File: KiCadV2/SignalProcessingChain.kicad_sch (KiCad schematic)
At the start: 29 parts, among them U10 NC7SZ157P6X, U11 NC7SZ157P6X, U12 NC7SZ157P6X, U13 NC7SZ157P6X, U14 74LV08AT14-13, U15 HIP4080A, U17 MX3502S, U8 NC7SZ157P6X, U9 NC7SZ157P6X

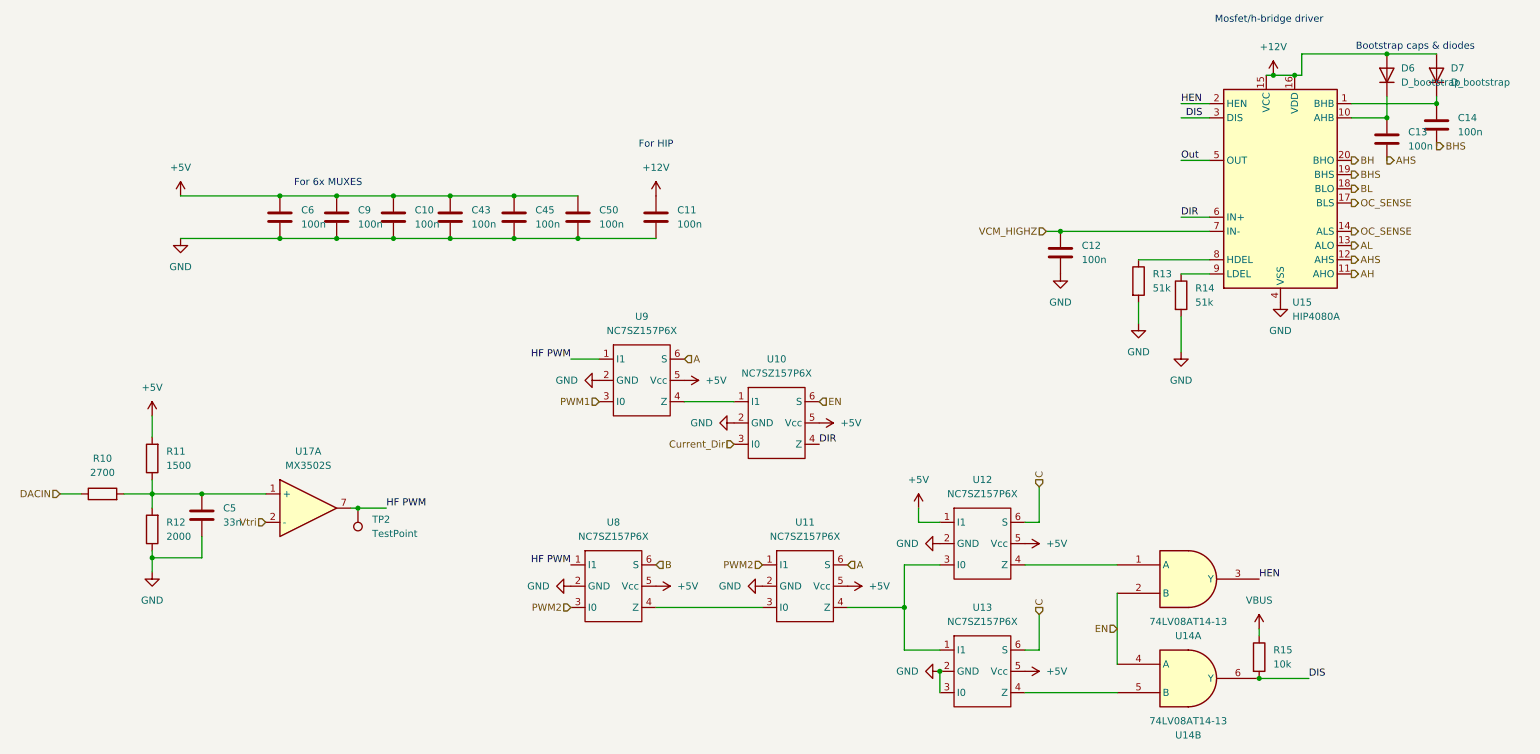
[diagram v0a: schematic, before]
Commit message: saving here before i try making PerCoilFlipped on schematic
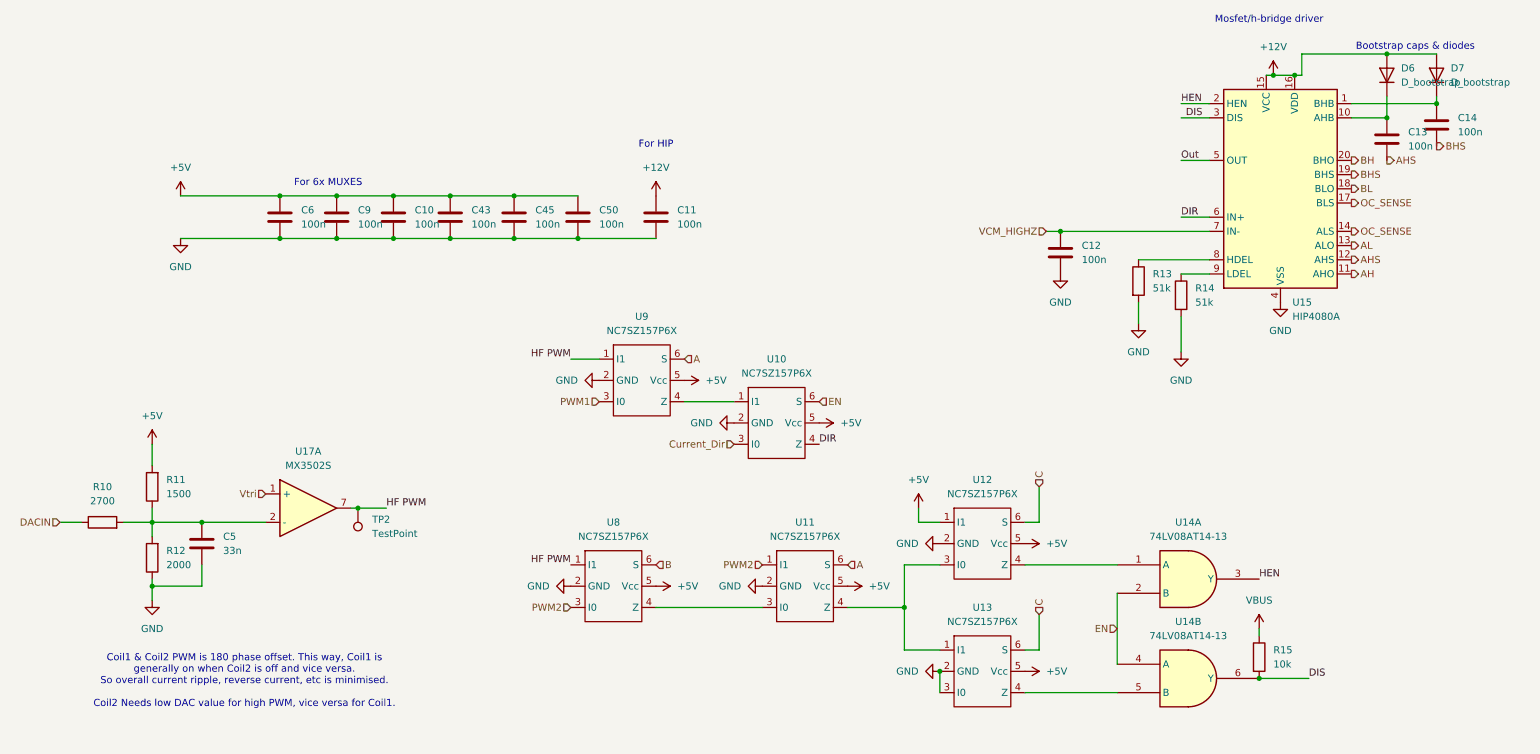
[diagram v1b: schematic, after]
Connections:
- net Vtri: now also U17.1 (+); no longer U17.2 (-)
- net at C5.1, R10.2, R11.1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: now also U17.2 (-); no longer U17.1 (+)
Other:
- note added: "Coil1 & Coil2 PWM is 180 phase offset. This way, Coil1 is generally on when Coil2 is off and vice versa. So overall current ripple, reverse current, etc is minimised. Coil2 Needs low DAC value for high PWM, vice versa for Coil1."
- moved on the sheet: C5, R10, R11, R12
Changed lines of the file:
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@@
 		)
 	)
+	(text "Coil1 & Coil2 PWM is 180 phase offset. This way, Coil1 is \ngenerally on when Coil2 is off and vice versa.\nSo overall current ripple, reverse current, etc is minimised.\n\nCoil2 Needs low DAC value for high PWM, vice versa for Coil1.\n\n"
+		(exclude_from_sim no)
+		(at 62.23 136.144 0)
+		(effects
+			(font
+				(size 1.27 1.27)
+			)
+		)
+	)
 	(text "Mosfet/h-bridge driver"
 		(exclude_from_sim no)
@@
 	)
 	(junction
-		(at 54.61 101.6)
-		(diameter 0)
-		(color 0 0 0 0)
-	)
-	(junction
 		(at 99.06 48.26)
 		(diameter 0)
@@
 	)
 	(junction
-		(at 45.72 101.6)
+		(at 45.72 106.68)
 		(diameter 0)
 		(color 0 0 0 0)
@@
 	)
 	(junction
-		(at 45.72 113.03)
+		(at 54.61 106.68)
+		(diameter 0)
+		(color 0 0 0 0)
+	)
+	(junction
+		(at 45.72 118.11)
 		(diameter 0)
 		(color 0 0 0 0)
@@
 	(wire
 		(pts
-			(xy 40.64 101.6) (xy 45.72 101.6)
+			(xy 40.64 106.68) (xy 45.72 106.68)
 		)
 		(stroke
@@
 	(wire
 		(pts
-			(xy 45.72 101.6) (xy 45.72 104.14)
+			(xy 45.72 106.68) (xy 45.72 109.22)
 		)
 		(stroke
@@
 	(wire
 		(pts
-			(xy 45.72 101.6) (xy 54.61 101.6)
+			(xy 45.72 106.68) (xy 54.61 106.68)
 		)
 		(stroke
@@
 	(wire
 		(pts
-			(xy 45.72 99.06) (xy 45.72 101.6)
+			(xy 45.72 104.14) (xy 45.72 106.68)
 		)
 		(stroke
@@
 	(wire
 		(pts
-			(xy 45.72 113.03) (xy 54.61 113.03)
+			(xy 45.72 118.11) (xy 54.61 118.11)
 		)
 		(stroke
@@
 	(wire
 		(pts
-			(xy 45.72 87.63) (xy 45.72 91.44)
+			(xy 45.72 92.71) (xy 45.72 96.52)
 		)
 		(stroke
@@
 	(wire
 		(pts
-			(xy 29.21 101.6) (xy 33.02 101.6)
+			(xy 29.21 106.68) (xy 33.02 106.68)
 		)
 		(stroke
@@
 	(wire
 		(pts
-			(xy 45.72 113.03) (xy 45.72 115.57)
+			(xy 45.72 118.11) (xy 45.72 120.65)
 		)
 		(stroke
@@
 	(wire
 		(pts
-			(xy 45.72 111.76) (xy 45.72 113.03)
+			(xy 45.72 116.84) (xy 45.72 118.11)
 		)
 		(stroke
@@
 	(wire
 		(pts
-			(xy 54.61 101.6) (xy 66.04 101.6)
+			(xy 54.61 106.68) (xy 66.04 106.68)
 		)
 		(stroke
@@
 	(wire
 		(pts
-			(xy 54.61 113.03) (xy 54.61 109.22)
+			(xy 54.61 118.11) (xy 54.61 114.3)
 		)
 		(stroke
@@
 	(hierarchical_label "DACIN"
 		(shape input)
-		(at 29.21 101.6 180)
+		(at 29.21 106.68 180)
 		(effects
 			(font
@@
 	(hierarchical_label "Vtri"
 		(shape input)
-		(at 66.04 106.68 180)
+		(at 66.04 101.6 180)
 		(fields_autoplaced yes)
 		(effects
@@
 		)
 		(property "Netclass" "HF"
-			(at 66.04 107.95 0)
+			(at 66.04 102.87 0)
 			(effects
 				(font
@@
 	(symbol
 		(lib_id "power:+5V")
-		(at 45.72 87.63 0)
+		(at 45.72 92.71 0)
 		(unit 1)
 		(exclude_from_sim no)
@@
 		(fields_autoplaced yes)
 		(property "Reference" "#PWR027"
-			(at 45.72 91.44 0)
+			(at 45.72 96.52 0)
 			(effects
 				(font
@@
 		)
 		(property "Value" "+5V"
-			(at 45.72 82.55 0)
+			(at 45.72 87.63 0)
 			(effects
 				(font
@@
 		)
 		(property "Footprint" ""
-			(at 45.72 87.63 0)
+			(at 45.72 92.71 0)
 			(effects
 				(font
@@
 		)
 		(property "Datasheet" ""
-			(at 45.72 87.63 0)
+			(at 45.72 92.71 0)
 			(effects
 				(font
@@
 		)
 		(property "Description" "Power symbol creates a global label with name \"+5V\""
-			(at 45.72 87.63 0)
+			(at 45.72 92.71 0)
 			(effects
 				(font
@@
 	(symbol
 		(lib_id "power:GND")
-		(at 45.72 115.57 0)
+		(at 45.72 120.65 0)
 		(unit 1)
 		(exclude_from_sim no)
@@
 		(fields_autoplaced yes)
 		(property "Reference" "#PWR028"
-			(at 45.72 121.92 0)
+			(at 45.72 127 0)
 			(effects
 				(font
@@
 		)
 		(property "Value" "GND"
-			(at 45.72 120.65 0)
+			(at 45.72 125.73 0)
 			(effects
 				(font
@@
 		)
 		(property "Footprint" ""
-			(at 45.72 115.57 0)
+			(at 45.72 120.65 0)
 			(effects
 				(font
@@
 		)
 		(property "Datasheet" ""
-			(at 45.72 115.57 0)
+			(at 45.72 120.65 0)
 			(effects
 				(font
@@
 		)
 		(property "Description" "Power symbol creates a global label with name \"GND\" , ground"
-			(at 45.72 115.57 0)
+			(at 45.72 120.65 0)
 			(effects
 				(font
@@
 		(fields_autoplaced yes)
 		(property "Reference" "U14"
-			(at 231.1511 127 0)
+			(at 231.151 106.68 0)
 			(effects
 				(font
@@
 		)
 		(property "Value" "74LV08AT14-13"
-			(at 231.1511 124.46 0)
+			(at 231.151 109.22 0)
 			(effects
 				(font
@@
 	(symbol
 		(lib_id "Device:R")
-		(at 36.83 101.6 90)
+		(at 36.83 106.68 90)
 		(unit 1)
 		(exclude_from_sim no)
@@
 		(fields_autoplaced yes)
 		(property "Reference" "R10"
-			(at 36.83 95.25 90)
+			(at 36.83 100.33 90)
 			(effects
 				(font
@@
 		)
 		(property "Value" "2700"
-			(at 36.83 97.79 90)
+			(at 36.83 102.87 90)
 			(effects
 				(font
@@
 		)
 		(property "Footprint" "Resistor_SMD:R_0603_1608Metric"
-			(at 36.83 103.378 90)
+			(at 36.83 108.458 90)
 			(effects
 				(font
@@
 		)
 		(property "Datasheet" "~"
-			(at 36.83 101.6 0)
+			(at 36.83 106.68 0)
 			(effects
 				(font
@@
 		)
 		(property "Description" "Resistor"
-			(at 36.83 101.6 0)
+			(at 36.83 106.68 0)
 			(effects
 				(font
@@
 		)
 		(property "LCSC" "C13167"
-			(at 36.83 101.6 0)
+			(at 36.83 106.68 0)
 			(effects
 				(font
@@
 	(symbol
 		(lib_id "Device:R")
-		(at 45.72 107.95 180)
+		(at 45.72 113.03 180)
 		(unit 1)
 		(exclude_from_sim no)
@@
 		(fields_autoplaced yes)
 		(property "Reference" "R12"
-			(at 48.26 106.6799 0)
+			(at 48.26 111.7599 0)
 			(effects
 				(font
@@
 		)
 		(property "Value" "2000"
-			(at 48.26 109.2199 0)
+			(at 48.26 114.2999 0)
 			(effects
 				(font
@@
 		)
 		(property "Footprint" "Resistor_SMD:R_0603_1608Metric"
-			(at 47.498 107.95 90)
+			(at 47.498 113.03 90)
 			(effects
 				(font
@@
 		)
 		(property "Datasheet" "~"
-			(at 45.72 107.95 0)
+			(at 45.72 113.03 0)
 			(effects
 				(font
@@
 		)
 		(property "Description" "Resistor"
-			(at 45.72 107.95 0)
+			(at 45.72 113.03 0)
 			(effects
 				(font
@@
 		)
 		(property "LCSC" "C22975"
-			(at 45.72 107.95 0)
+			(at 45.72 113.03 0)
 			(effects
 				(font
@@
 	(symbol
 		(lib_id "Device:C")
-		(at 54.61 105.41 0)
+		(at 54.61 110.49 0)
 		(unit 1)
 		(exclude_from_sim no)
@@
 		(fields_autoplaced yes)
 		(property "Reference" "C5"
-			(at 58.42 104.1399 0)
+			(at 58.42 109.2199 0)
 			(effects
 				(font
@@
 		)
 		(property "Value" "33n"
-			(at 58.42 106.6799 0)
+			(at 58.42 111.7599 0)
 			(effects
 				(font
@@
 		)
 		(property "Footprint" "Capacitor_SMD:C_0603_1608Metric"
-			(at 55.5752 109.22 0)
+			(at 55.5752 114.3 0)
 			(effects
 				(font
@@
 		)
 		(property "Datasheet" "~"
-			(at 54.61 105.41 0)
+			(at 54.61 110.49 0)
 			(effects
 				(font
@@
 		)
 		(property "Description" "Unpolarized capacitor"
-			(at 54.61 105.41 0)
+			(at 54.61 110.49 0)
 			(effects
 				(font
@@
 		)
 		(property "LCSC" "C21117"
-			(at 54.61 105.41 0)
+			(at 54.61 110.49 0)
 			(effects
 				(font
@@
 	(symbol
 		(lib_id "Device:R")
-		(at 45.72 95.25 180)
+		(at 45.72 100.33 180)
 		(unit 1)
 		(exclude_from_sim no)
@@
 		(fields_autoplaced yes)
 		(property "Reference" "R11"
-			(at 48.26 93.9799 0)
+			(at 48.26 99.0599 0)
 			(effects
 				(font
@@
 		)
 		(property "Value" "1500"
-			(at 48.26 96.5199 0)
+			(at 48.26 101.5999 0)
 			(effects
 				(font
@@
 		)
 		(property "Footprint" "Resistor_SMD:R_0603_1608Metric"
-			(at 47.498 95.25 90)
+			(at 47.498 100.33 90)
 			(effects
 				(font
@@
 		)
 		(property "Datasheet" "~"
-			(at 45.72 95.25 0)
+			(at 45.72 100.33 0)
 			(effects
 				(font
@@
 		)
 		(property "Description" "Resistor"
-			(at 45.72 95.25 0)
+			(at 45.72 100.33 0)
 			(effects
 				(font
@@
 		)
 		(property "LCSC" "C22843"
-			(at 45.72 95.25 0)
+			(at 45.72 100.33 0)
 			(effects
 				(font
@@
 		(fields_autoplaced yes)
 		(property "Reference" "U14"
-			(at 231.1511 144.78 0)
+			(at 231.151 124.46 0)
 			(effects
 				(font
@@
 		)
 		(property "Value" "74LV08AT14-13"
-			(at 231.1511 142.24 0)
+			(at 231.151 127 0)
 			(effects
 				(font
